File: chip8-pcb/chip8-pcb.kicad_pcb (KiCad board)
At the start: 4 copper layers, 80 x 125 mm, 68 parts, among them J3 Battery, J4 Matrix Keypad, J5 Display, Q1 S8050, Q2 BCM857BS, Q3 CJ2301, SW1 SHDN, U1 TP5400, U2 AP2112K-3.3, U3 W25Q128JVS, U4 ESP32-C3-ZERO

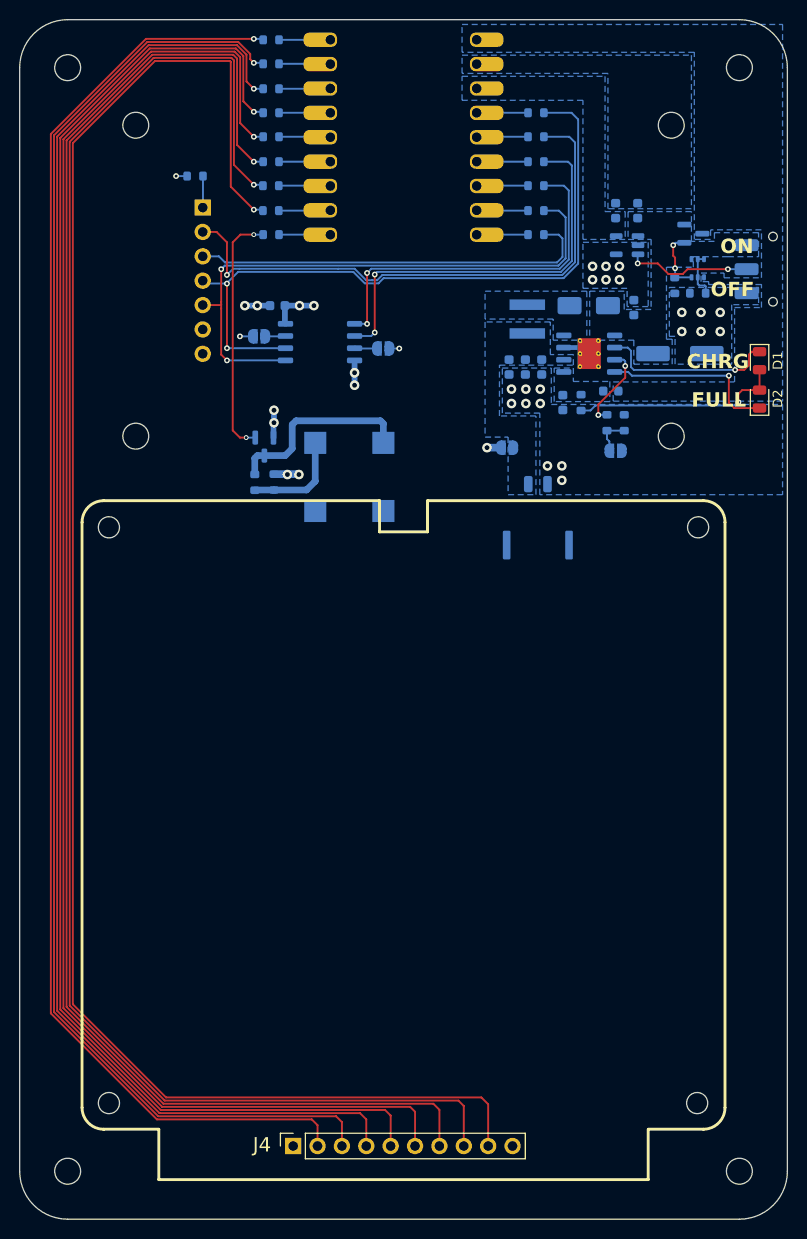
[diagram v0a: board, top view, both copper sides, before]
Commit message: chip8-pcb: final v2 version
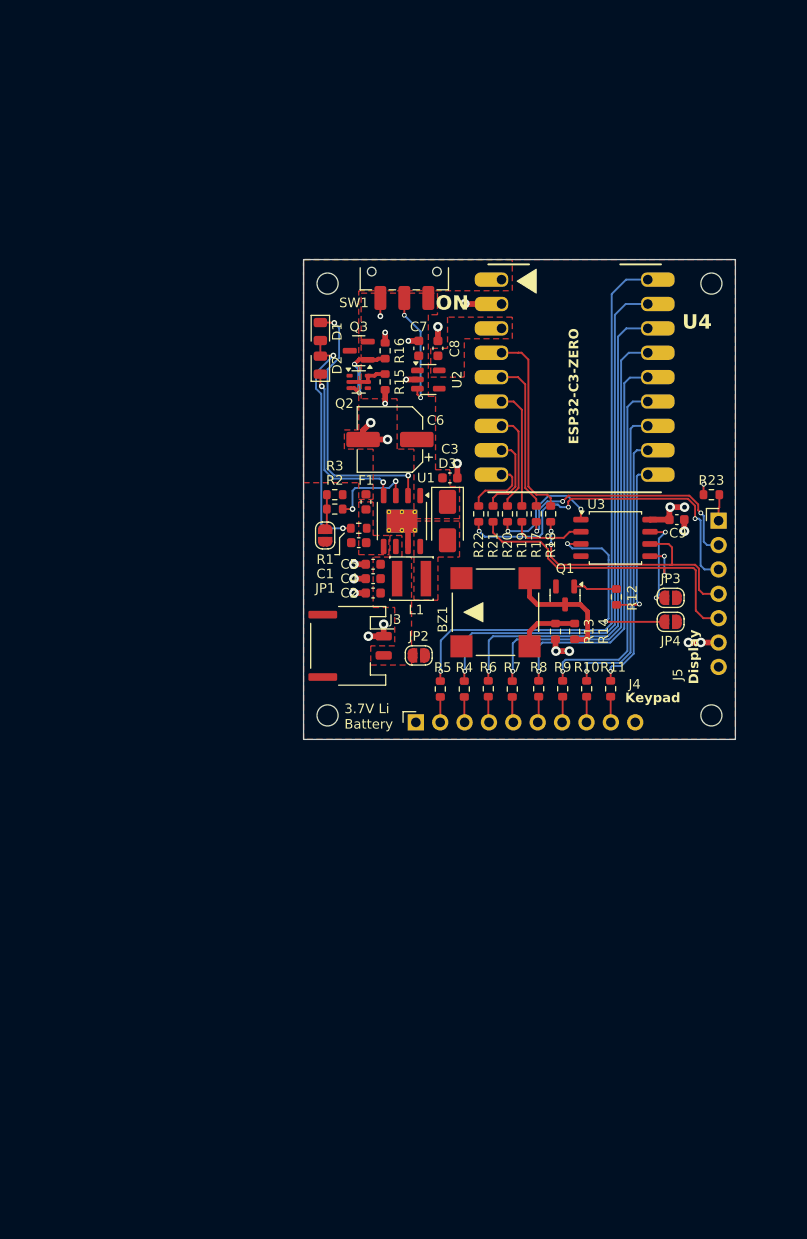
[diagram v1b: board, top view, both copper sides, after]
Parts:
- removed H1, H2, H3, H4: ~, MountingHole:MountingHole_2.7mm_M2.5
- removed H5, H6, H7, H8: ~, MountingHole:MountingHole_2.2mm_M2
- removed REF**: OSHW-Logo2_7.3x6mm_SilkScreen, Symbol:OSHW-Logo2_7.3x6mm_SilkScreen
- removed REF**: KiCad-Logo2_5mm_SilkScreen, Symbol:KiCad-Logo2_5mm_SilkScreen
- BZ1, C1, C2, C3, C4, C5, C6, C7, C8, C9, D3, F1, J3, J5, JP1, JP2, JP3, JP4, L1, Q1, Q2, Q3, R1, R10, R11, R12, R13, R14, R15, R16, R17, R18, R19, R2, R20, R21, R22, R23, R3, R4, R5, R6, R7, R8, R9, SW1, U1, U2, U3, U4: moved to F.Cu
- H10, H11, H12, H9: footprint MountingHole:MountingHole_2.7mm_M2.5 -> MountingHole:MountingHole_2.2mm_M2
- J4: footprint chip8-pcb:AZDelivery_Keypad_4x4_Matrix_P2.54mm -> Connector_PinSocket_2.54mm:PinSocket_1x10_P2.54mm_Horizontal
- moved H12 82.2 mm to (112.1, 117.5)
- moved H9 70.8 mm to (112.1, 72.5)
- moved R5 69.9 mm to (83.8, 114.8), turned to -90 degrees
- moved R4 68.2 mm to (86.3, 114.8), turned to -90 degrees
- moved R6 66.5 mm to (88.8, 114.7), turned to -90 degrees
- moved R7 65.1 mm to (91.3, 114.8), turned to -90 degrees
- moved H11 64.0 mm to (72.1, 117.5)
- moved R8 63.9 mm to (94.1, 114.7), turned to -90 degrees
- moved R23 63.2 mm to (112.1, 94.5)
- moved J5 62.9 mm to (112.8, 97.2), turned to 0 degrees
- moved R9 62.8 mm to (96.6, 114.7), turned to -90 degrees
- moved R10 61.9 mm to (99.1, 114.7), turned to -90 degrees
- moved R11 61.1 mm to (101.6, 114.7), turned to -90 degrees
- moved R12 52.2 mm to (102.2, 105.2), turned to 90 degrees
- moved JP3 50.8 mm to (107.8, 105.2), turned to 180 degrees
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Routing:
- net Net-(J4-C4): track 179.1 -> 2.68 mm, vias 1 -> 0
- net Net-(J4-C3): track 175.2 -> 2.68 mm, vias 1 -> 0
- net Net-(J4-C2): track 171.4 -> 2.70 mm, vias 1 -> 0
- net Net-(J4-C1): track 167.5 -> 2.72 mm, vias 1 -> 0
- net Net-(J4-R4): track 163.6 -> 2.70 mm, vias 1 -> 0
- net Net-(J4-R3): track 159.7 -> 2.70 mm, vias 1 -> 0
- net Net-(J4-R2): track 155.8 -> 2.66 mm, vias 1 -> 0
- net Net-(J4-R1): track 152.7 -> 2.65 mm, vias 1 -> 0
- net Net-(U4-GP21): track 5.36 -> 61.5 mm, vias 0 -> 1
- net Net-(U4-GP20): track 5.37 -> 56.8 mm, vias 0 -> 1
- net Net-(U4-GP19): track 5.37 -> 51.9 mm, vias 0 -> 1
- net SCLK: track 72.9 -> 28.3 mm
- net Net-(U4-GP18): track 5.36 -> 46.9 mm, vias 0 -> 1
- net Net-(U4-GP10): track 5.38 -> 41.6 mm, vias 0 -> 1
- net MISO: track 42.5 -> 7.77 mm, vias 2 -> 0
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- added copper zone on F.Cu, net +3.3V
- added copper zone on F.Cu, net +5V
- added copper zone on F.Cu, net +BATT
- added copper zone on F.Cu, net GND
- added copper zone on F.Cu, net Net-(D3-A)
- added copper zone on F.Cu, net Net-(U1-VCC)
- added copper zone on F.Cu, net VBUS
- removed copper zone on B.Cu, net +3.3V
- removed copper zone on B.Cu, net +5V
- removed copper zone on B.Cu, net +BATT
- removed copper zone on B.Cu, net GND
- removed copper zone on B.Cu, net Net-(D3-A)
- removed copper zone on B.Cu, net Net-(U1-VCC)
- removed copper zone on B.Cu, net VBUS
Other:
- board size 80 x 125 mm -> 45 x 50 mm
- board text added: "3.7V Li Battery"
- board text added: "Display"
- board text added: "ESP32-C3-ZERO"
- board text added: "Keypad"
- board text added: "Rev. 1"
- board text removed: "CHRG"
- board text removed: "FULL"
- board text removed: "LiPo / Li-Ion Battery (3.7V)"
- board text removed: "OFF"
